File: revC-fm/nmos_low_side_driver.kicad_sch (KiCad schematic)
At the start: 6 parts, among them Q49 MMDT3946, Q57 MMBT2907AM3T5G

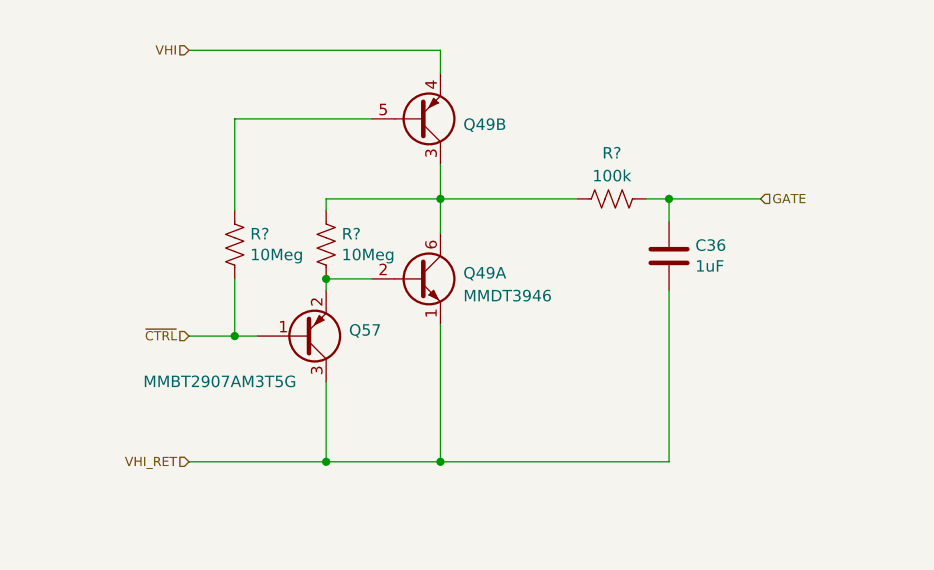
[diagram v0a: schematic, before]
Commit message: working revC review changes
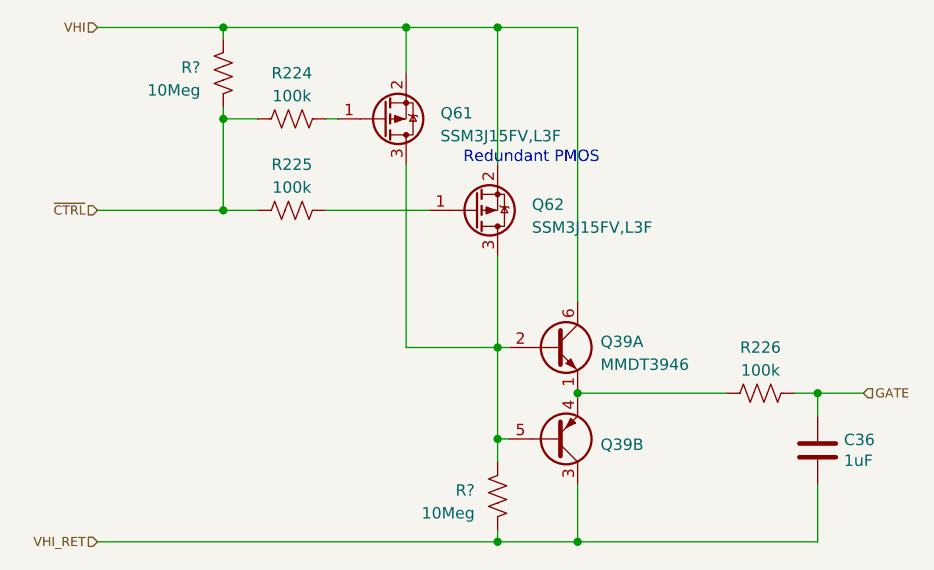
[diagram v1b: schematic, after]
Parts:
- removed Q49: MMDT3946, Package_TO_SOT_SMD:SOT-363_SC-70-6, symbol Transistor_BJT:MMDT3946
- removed Q57: MMBT2907AM3T5G, SierraLobo:SOT-723, symbol Device:Q_PNP_BEC
- removed R?: 10Meg, Resistor_SMD:R_0603_1608Metric, symbol Device:R_US
- removed R?: 100k, Resistor_SMD:R_0603_1608Metric, symbol Device:R_US
- added Q39: MMDT3946, Package_TO_SOT_SMD:SOT-363_SC-70-6, symbol Transistor_BJT:MMDT3946
- added Q61, Q62: SSM3J15FV,L3F, Package_TO_SOT_SMD:SOT-723, symbol Device:Q_PMOS_GSD
- added R224, R225, R226: 100k, Resistor_SMD:R_0603_1608Metric, symbol Device:R_US
- added R?: 10Meg, Resistor_SMD:R_0603_1608Metric, symbol Device:R_US
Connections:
- net GATE: now also R226.2
- net VHI: now also R?.1, Q39.6 (C1), Q61.2 (S), Q62.2 (S)
- net VHI_RET: now also Q39.3 (C2), R?.2
- net ~{CTRL}: now also R224.1, R225.1
- new net: Q62.1 (G), R225.2
- new net: Q39.1 (E1), Q39.4 (E2), R226.1
- new net: Q39.2 (B1), Q39.5 (B2), Q61.3 (D), Q62.3 (D), R?.1
- new net: Q61.1 (G), R224.2
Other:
- note added: "Redundant PMOS"
- moved on the sheet: C36, R?
